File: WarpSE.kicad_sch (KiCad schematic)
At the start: 9 parts

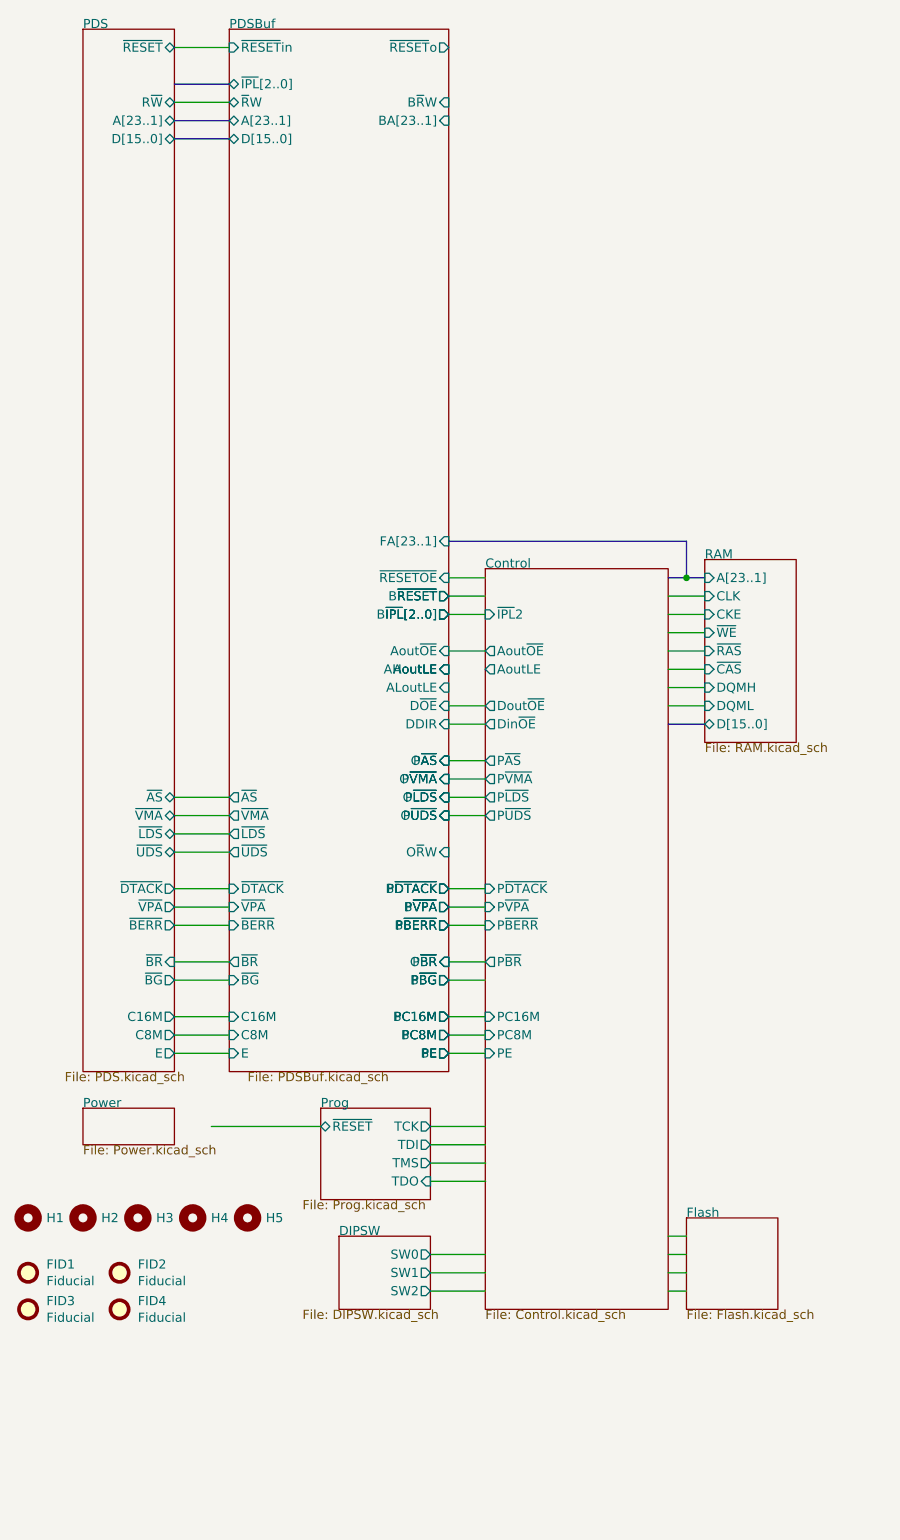
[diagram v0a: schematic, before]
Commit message: more
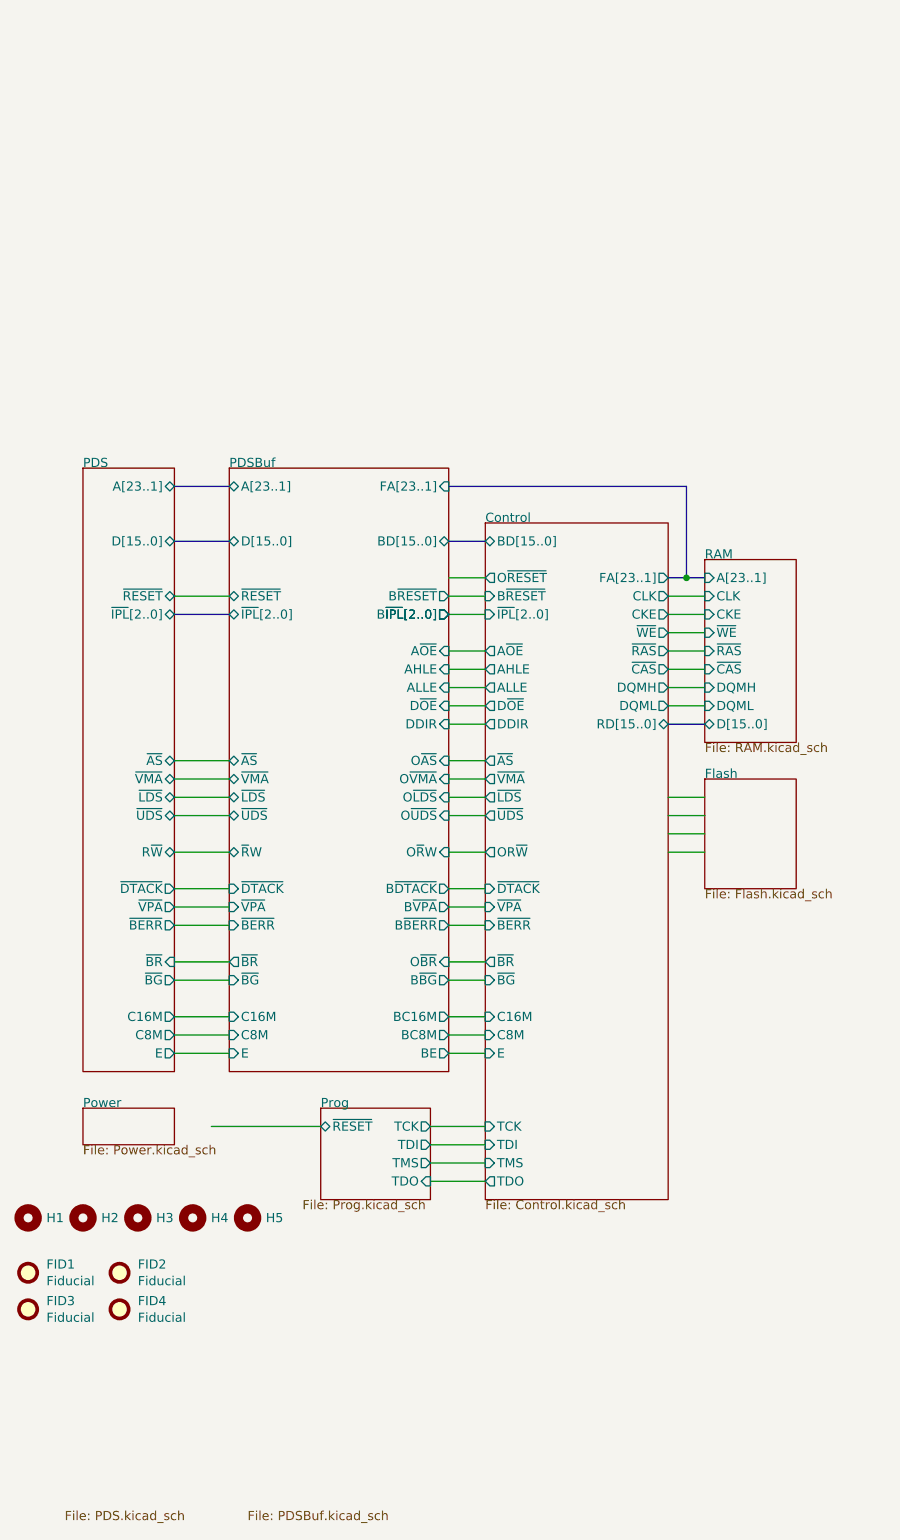
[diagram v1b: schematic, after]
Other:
- removed sheet DIPSW
- sheet Control ports: added AHLE, ALLE, A~{OE}, BD[15..0], B~{RESET}, C16M, C8M, CKE, CLK, DDIR, DQMH, DQML, D~{OE}, E, FA[23..1], OR~{W}, O~{RESET}, RD[15..0], TCK, TDI, TDO, TMS, ~{AS}, ~{BERR}, ~{BG}, ~{BR}, ~{CAS}, ~{DTACK}, ~{IPL}[2..0], ~{LDS}, ~{RAS}, ~{UDS}, ~{VMA}, ~{VPA}, ~{WE}; removed AoutLE, Aout~{OE}, Din~{OE}, Dout~{OE}, PC16M, PC8M, PE, P~{AS}, P~{BERR}, P~{BR}, P~{DTACK}, P~{LDS}, P~{UDS}, P~{VMA}, P~{VPA}, ~{IPL}2
- sheet PDS ports: added ~{IPL}[2..0]; removed none
- sheet PDSBuf ports: added AHLE, ALLE, A~{OE}, BD[15..0]; removed AHoutLE, ALoutLE, AoutLE, Aout~{OE}, BA[23..1], B~{R}W, PC16M, PC8M, PE, P~{AS}, P~{BERR}, P~{BG}, P~{BR}, P~{DTACK}, P~{LDS}, P~{UDS}, P~{VMA}, P~{VPA}, ~{RESETOE}, ~{RESET}in, ~{RESET}o
